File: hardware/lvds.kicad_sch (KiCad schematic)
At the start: 52 parts, among them U4 GateMate-CCGM1A1, Y1 ASE2-25.000MHZ-L-C-T

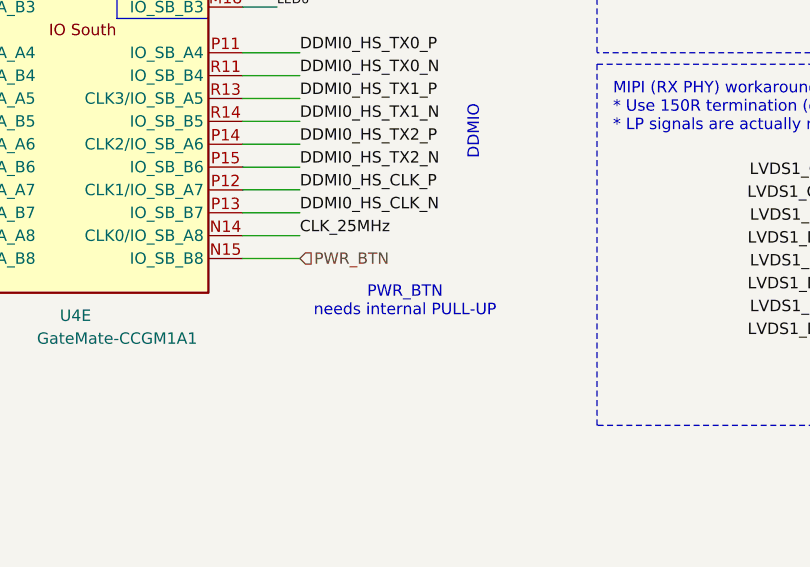
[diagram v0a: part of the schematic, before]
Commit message: CleanUP
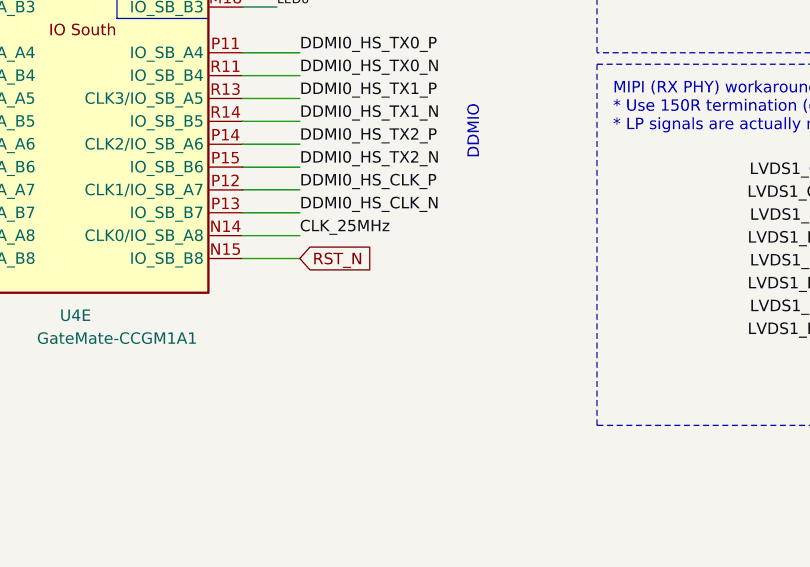
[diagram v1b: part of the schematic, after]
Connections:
- net PWR_BTN renamed RST_N
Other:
- note removed: "PWR_BTN needs internal PULL-UP"
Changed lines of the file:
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@@
 		)
 	)
-	(text "PWR_BTN\nneeds internal PULL-UP"
-		(exclude_from_sim no)
-		(at 188.214 106.426 0)
-		(effects
-			(font
-				(size 1.27 1.27)
-			)
-		)
-	)
 	(junction
 		(at 119.38 38.1)
@@
 		)
 	)
+	(global_label "RST_N"
+		(shape input)
+		(at 176.53 101.6 0)
+		(fields_autoplaced yes)
+		(effects
+			(font
+				(size 1.27 1.27)
+			)
+			(justify left)
+		)
+		(property "Intersheetrefs" "${INTERSHEET_REFS}"
+			(at 185.2604 101.6 0)
+			(effects
+				(font
+					(size 1.27 1.27)
+				)
+				(justify left)
+				(hide yes)
+			)
+		)
+	)
 	(hierarchical_label "{LVDS1}"
 		(shape bidirectional)
@@
 		)
 	)
-	(hierarchical_label "PWR_BTN"
-		(shape input)
-		(at 176.53 101.6 0)
-		(effects
-			(font
-				(size 1.254 1.254)
-			)
-			(justify left)
-		)
-	)
